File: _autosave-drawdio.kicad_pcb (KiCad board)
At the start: 2 copper layers, 45.7 x 12.7 mm, 12 parts, among them P1 CONN_2, P2 CONN_01X01, Q1 BC558, Q2 BC547, U1 LM555N

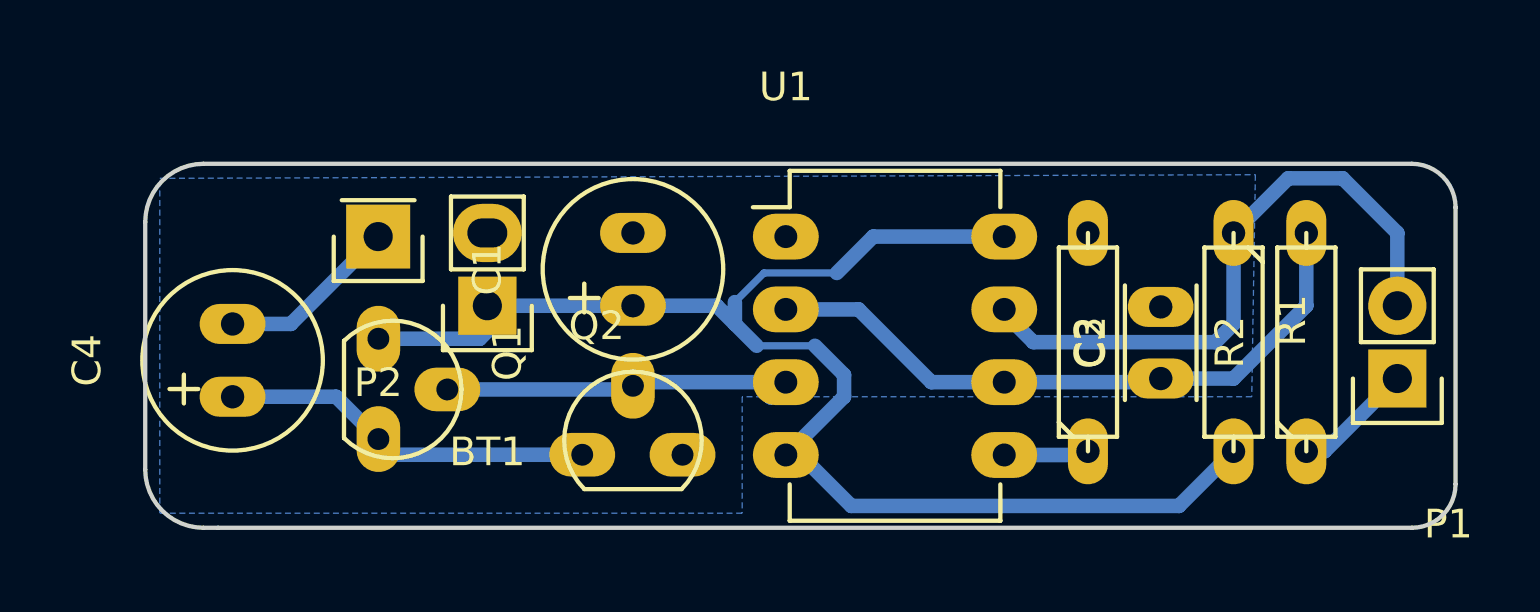
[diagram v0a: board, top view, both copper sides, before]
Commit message: V0.2
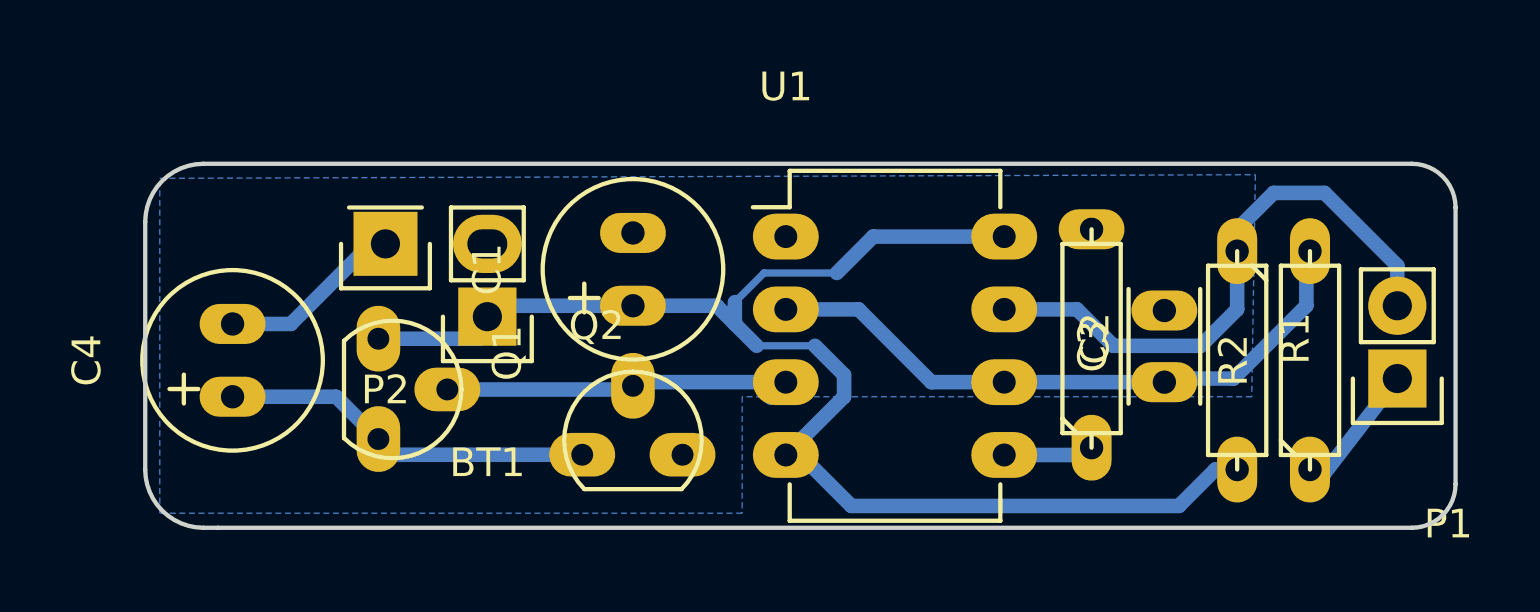
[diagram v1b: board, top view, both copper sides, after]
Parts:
- moved R1 0.65 mm to (121.4, 87.6)
- moved R2 0.65 mm to (118.9, 87.6)
- moved BT1 0.38 mm to (92.7, 86.1)
- moved P2 0.36 mm to (89.2, 83.6)
- moved C2 0.18 mm to (113.8, 86.9)
- moved C3 0.18 mm to (116.3, 88.4)
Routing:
- net Net-(P1-Pad2): track 21.8 -> 20.8 mm
- net Net-(C3-Pad1): track 23.6 -> 22.9 mm
- net Net-(P1-Pad1): track 4.23 -> 4.80 mm
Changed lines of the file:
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@@
   (general
     (links 22)
-    (no_connects 1)
-    (area 80.696999 80.696999 126.567001 93.547001)
+    (no_connects 0)
+    (area 71.10662 76.913 127.717572 97.536)
     (thickness 1.6)
     (drawings 11)
-    (tracks 58)
+    (tracks 60)
     (zones 0)
     (modules 12)
@@
     (mod_text_size 1 1)
     (mod_text_width 0.15)
-    (pad_size 2.4 2.032)
-    (pad_drill 1.4)
+    (pad_size 2.3 1.397)
+    (pad_drill 0.8128)
     (pad_to_mask_clearance 0)
     (aux_axis_origin 0 0)
@@
   )
   (module Pin_Headers:Pin_Header_Straight_1x02 (layer F.Cu)
-    (at 92.71 85.725 180)
+    (at 92.71 86.106 180)
     (descr "Through hole pin header")
     (tags "pin header")
@@
   )
   (module Capacitors_ThroughHole:C_Rect_L4_W2.5_P2.5 (layer F.Cu)
-    (at 116.205 88.265 90)
+    (at 116.332 88.392 90)
     (descr "Film Capacitor Length 4mm x Width 2.5mm, Pitch 2.5mm")
     (tags Capacitor)
@@
   )
   (module Discret:R3 (layer F.Cu)
-    (at 121.285 86.995 90)
+    (at 121.412 87.63 90)
     (descr "Resitance 3 pas")
     (tags R)
@@
   )
   (module Discret:R3 (layer F.Cu)
-    (at 118.745 86.995 270)
+    (at 118.872 87.63 270)
     (descr "Resitance 3 pas")
     (tags R)
@@
   )
   (module Discret:R3 (layer F.Cu)
-    (at 113.665 86.995 90)
+    (at 113.792 86.868 90)
     (descr "Resitance 3 pas")
     (tags R)
@@
     (pad 1 thru_hole oval (at -3.81 0 90) (size 2.3 1.397) (drill 0.8128) (layers *.Cu *.Mask F.SilkS)
       (net 3 "Net-(C2-Pad1)"))
-    (pad 2 thru_hole oval (at 3.81 0 90) (size 2.3 1.397) (drill 0.8128) (layers *.Cu *.Mask F.SilkS)
+    (pad 2 thru_hole oval (at 3.81 0 180) (size 2.3 1.397) (drill 0.8128) (layers *.Cu *.Mask F.SilkS)
       (net 1 GND))
     (model Discret.3dshapes/R3.wrl
@@
   )
   (module Pin_Headers:Pin_Header_Straight_1x01 (layer F.Cu)
-    (at 88.9 83.312 180)
+    (at 89.154 83.566 180)
     (descr "Through hole pin header")
     (tags "pin header")
@@
     (arrow2b (pts (xy 76.708 92.964) (xy 76.121579 91.837496)))
   )
+  (segment (start 118.872 91.44) (end 118.11 91.44) (width 0.508) (layer B.Cu) (net 2))
+  (segment (start 105.41 92.71) (end 116.84 92.71) (width 0.508) (layer B.Cu) (net 2))
+  (segment (start 105.41 92.71) (end 103.632 90.932) (width 0.508) (layer B.Cu) (net 2))
+  (segment (start 118.11 91.44) (end 116.84 92.71) (width 0.508) (layer B.Cu) (net 2))
   (segment (start 92.71 85.725) (end 92.71 86.614) (width 0.508) (layer B.Cu) (net 2))
   (segment (start 92.71 86.614) (end 92.448 86.876) (width 0.508) (layer B.Cu) (net 2))
@@
   (segment (start 92.71 85.725) (end 92.075 86.36) (width 0.508) (layer B.Cu) (net 2))
   (segment (start 103.124 90.932) (end 103.632 90.932) (width 0.508) (layer B.Cu) (net 2))
-  (segment (start 103.632 90.932) (end 105.41 92.71) (width 0.508) (layer B.Cu) (net 2))
-  (segment (start 116.84 92.71) (end 118.745 90.805) (width 0.508) (layer B.Cu) (net 2))
-  (segment (start 105.41 92.71) (end 116.84 92.71) (width 0.508) (layer B.Cu) (net 2))
   (segment (start 110.744 83.312) (end 106.172 83.312) (width 0.508) (layer B.Cu) (net 2))
   (segment (start 101.346 85.598) (end 101.346 86.36) (width 0.508) (layer B.Cu) (net 2))
@@
   (segment (start 116.205 88.265) (end 118.745 88.265) (width 0.508) (layer B.Cu) (net 4))
   (segment (start 118.745 88.265) (end 121.285 85.725) (width 0.508) (layer B.Cu) (net 4))
-  (segment (start 121.285 85.725) (end 121.285 83.185) (width 0.508) (layer B.Cu) (net 4))
+  (segment (start 121.285 85.725) (end 121.285 83.947) (width 0.508) (layer B.Cu) (net 4) (status 20))
   (segment (start 110.744 88.392) (end 108.204 88.392) (width 0.508) (layer B.Cu) (net 4))
   (segment (start 105.664 85.852) (end 103.124 85.852) (width 0.508) (layer B.Cu) (net 4))
@@
   (segment (start 89.456 90.924) (end 87.432 88.9) (width 0.508) (layer B.Cu) (net 6))
   (segment (start 87.432 88.9) (end 83.82 88.9) (width 0.508) (layer B.Cu) (net 6))
-  (segment (start 121.285 90.805) (end 121.92 90.805) (width 0.508) (layer B.Cu) (net 7))
-  (segment (start 121.92 90.805) (end 124.46 88.265) (width 0.508) (layer B.Cu) (net 7))
-  (segment (start 118.745 83.185) (end 120.65 81.28) (width 0.508) (layer B.Cu) (net 8))
-  (segment (start 124.46 83.185) (end 124.46 85.725) (width 0.508) (layer B.Cu) (net 8))
-  (segment (start 122.555 81.28) (end 124.46 83.185) (width 0.508) (layer B.Cu) (net 8))
-  (segment (start 120.65 81.28) (end 122.555 81.28) (width 0.508) (layer B.Cu) (net 8))
-  (segment (start 118.745 83.185) (end 118.745 86.36) (width 0.508) (layer B.Cu) (net 8))
-  (segment (start 111.76 86.995) (end 110.744 85.979) (width 0.508) (layer B.Cu) (net 8))
-  (segment (start 118.11 86.995) (end 111.76 86.995) (width 0.508) (layer B.Cu) (net 8))
-  (segment (start 118.745 86.36) (end 118.11 86.995) (width 0.508) (layer B.Cu) (net 8))
+  (segment (start 121.285 91.567) (end 121.92 91.567) (width 0.508) (layer B.Cu) (net 7) (status 30))
+  (segment (start 121.92 91.567) (end 124.46 88.265) (width 0.508) (layer B.Cu) (net 7) (status 10))
+  (segment (start 110.744 85.852) (end 113.284 85.852) (width 0.508) (layer B.Cu) (net 8))
+  (segment (start 118.872 85.852) (end 118.872 83.058) (width 0.508) (layer B.Cu) (net 8))
+  (segment (start 117.602 87.122) (end 118.872 85.852) (width 0.508) (layer B.Cu) (net 8))
+  (segment (start 114.554 87.122) (end 117.602 87.122) (width 0.508) (layer B.Cu) (net 8))
+  (segment (start 113.284 85.852) (end 114.554 87.122) (width 0.508) (layer B.Cu) (net 8))
+  (segment (start 118.745 83.185) (end 120.142 81.788) (width 0.508) (layer B.Cu) (net 8))
+  (segment (start 124.46 84.328) (end 124.46 85.725) (width 0.508) (layer B.Cu) (net 8))
+  (segment (start 121.92 81.788) (end 124.46 84.328) (width 0.508) (layer B.Cu) (net 8))
+  (segment (start 120.142 81.788) (end 121.92 81.788) (width 0.508) (layer B.Cu) (net 8))
   (segment (start 110.744 85.979) (end 110.744 85.852) (width 0.508) (layer B.Cu) (net 8))
   (segment (start 97.663 88.646) (end 91.313 88.646) (width 0.508) (layer B.Cu) (net 9))
